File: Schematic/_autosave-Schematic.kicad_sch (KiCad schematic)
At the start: 17 parts, among them Q1 PMOS, Q2 PMOS, Q3 PMOS, Q4 PMOS, Q5 NMOS, Q6 NMOS, Q7 NMOS, Q8 NMOS, U1 TMC262

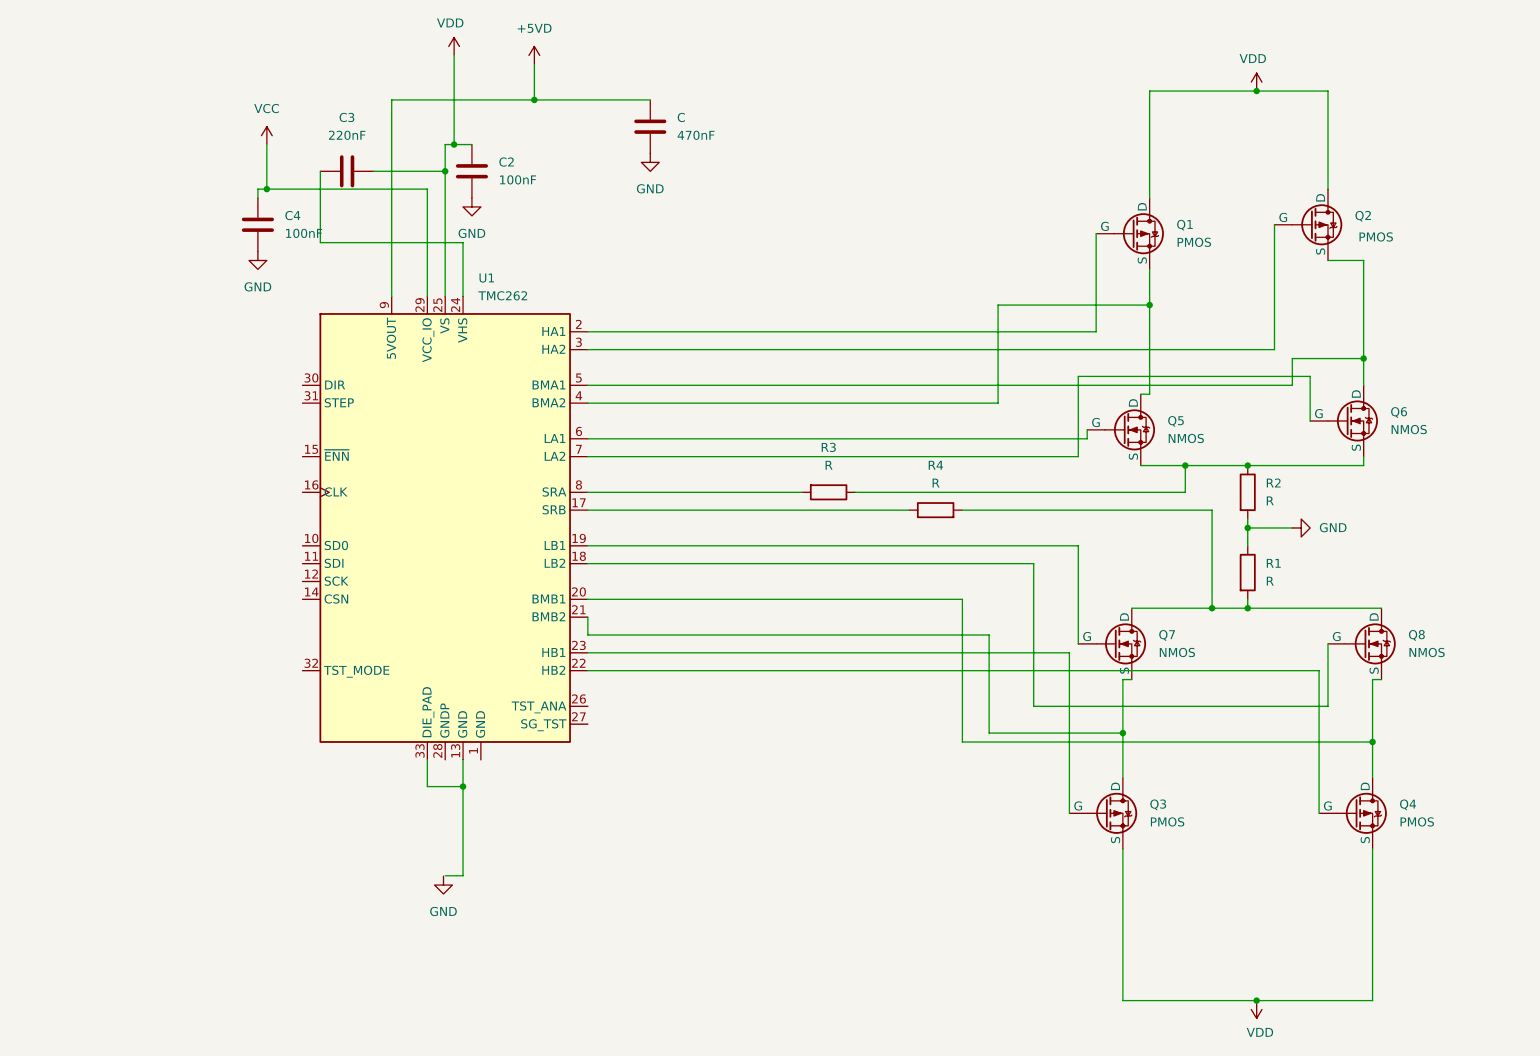
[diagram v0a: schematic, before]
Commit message: working on some stuff
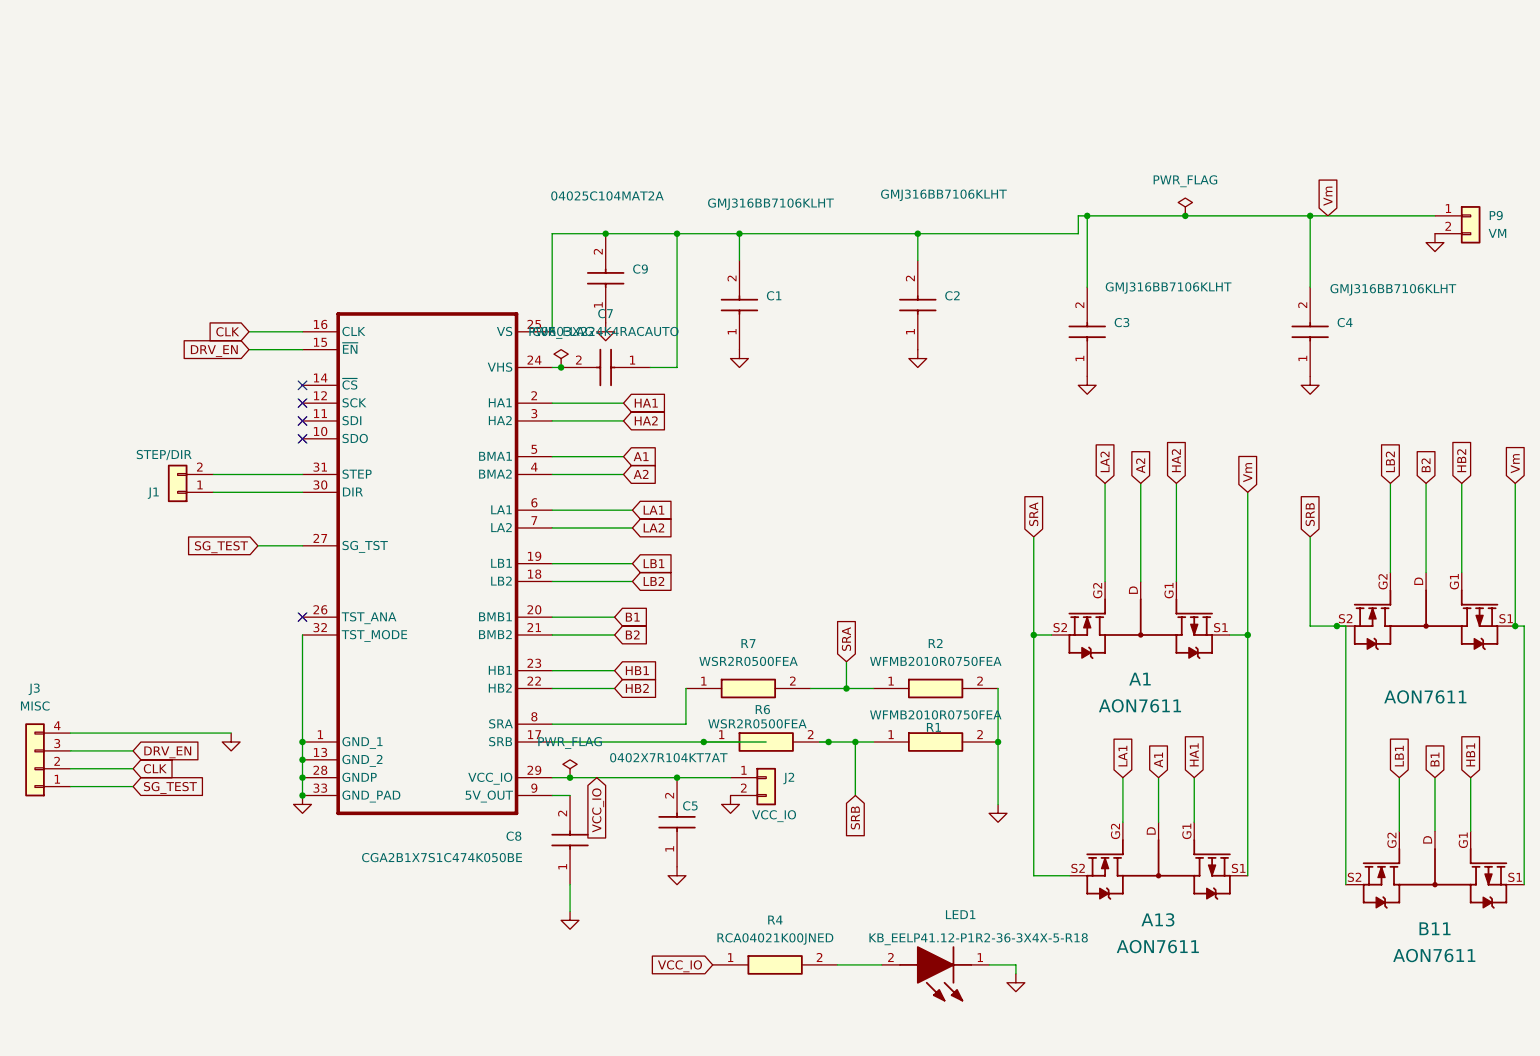
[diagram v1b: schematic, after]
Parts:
- removed C: 470nF, symbol Device:C
- removed C2, C4: 100nF, symbol Device:C
- removed C3: 220nF, symbol Device:C
- removed Q1, Q2, Q3, Q4: PMOS, symbol Simulation_SPICE:PMOS
- removed Q5, Q6, Q7, Q8: NMOS, symbol Simulation_SPICE:NMOS
- removed R1, R2, R3, R4: R, symbol Device:R
- removed U1: TMC262, Package_DFN_QFN:QFN-32-1EP_5x5mm_P0.5mm_EP3.45x3.45mm, symbol Driver_Motor:TMC262
- added A1, A13, B1, B11: AON7611, AON7611, symbol TMC262_BOB40_V1_2:AON7611
- added C1, C2, C3, C4: GMJ316BB7106KLHT, CAPPC3216X125N, symbol GMJ316BB7106KLHT:GMJ316BB7106KLHT
- added C5: 0402X7R104KT7AT, CAPC1005X61N, symbol 0402X7R104KT7AT:0402X7R104KT7AT
- added C7: C0603X224K4RACAUTO, C0603, symbol C0603X224K4RACAUTO:C0603X224K4RACAUTO
- added C8: CGA2B1X7S1C474K050BE, CAPC1005X55N, symbol CGA2B1X7S1C474K050BE:CGA2B1X7S1C474K050BE
- added C9: 04025C104MAT2A, CAPC1005X56N, symbol 04025C104MAT2A:04025C104MAT2A
- added IC1: ~, TMC262-LA:TMC_QFN32_0.5_5.0X5.0, symbol TMC262-LA:TMC262-LA
- added J1: STEP/DIR, symbol Connector_Generic:Conn_01x02
- added J2: VCC_IO, symbol Connector_Generic:Conn_01x02
- added J3: MISC, symbol Connector_Generic:Conn_01x04
- added LED1: KB_EELP41.12-P1R2-36-3X4X-5-R18, KBEELP4112P1R2363X4X5R18, symbol KB_EELP41_12-P1R2-36-3X4X-5-R1:KB_EELP41.12-P1R2-36-3X4X-5-R18
- added P9: VM, symbol Connector_Generic:Conn_01x02
- added R1, R2: WFMB2010R0750FEA, RESC5125X65N, symbol WFMB2010R0750FEA:WFMB2010R0750FEA
- added R4: RCA04021K00JNED, RESC1005X40N, symbol RCA04021K00JNED:RCA04021K00JNED
- added R6, R7: WSR2R0500FEA, RESM11670X254N, symbol WSR2R0500FEA:WSR2R0500FEA
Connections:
- net GND: now also C1.1, C2.1, C3.1, C4.1, C5.1, C8.1, C9.1, IC1.1 (GND_1), IC1.13 (GND_2), IC1.28 (GNDP), IC1.32 (TST_MODE), IC1.33 (GND_PAD), J2.2 (Pin_2), J3.4 (Pin_4), LED1.1 (K), P9.2 (Pin_2), R1.2, R2.2
- new net: C7.2, IC1.24 (VHS)
- new net: IC1.8 (SRA), R7.1
- new net: IC1.17 (SRB), R6.1
- new net: IC1.30 (DIR), J1.1 (Pin_1)
- new net: IC1.31 (STEP), J1.2 (Pin_2)
- new net: C8.2, IC1.9 (5V_OUT)
- new net: LED1.2 (A), R4.2
- new net A1: A13.D, IC1.5 (BMA1)
- new net A2: A1.D, IC1.4 (BMA2)
- new net B1: B11.D, IC1.20 (BMB1)
- new net B2: B1.D, IC1.21 (BMB2)
- new net CLK: IC1.16 (CLK), J3.2 (Pin_2)
- new net DRV_EN: IC1.15 (~{EN}), J3.3 (Pin_3)
- new net HA1: A13.G1, IC1.2 (HA1)
- new net HA2: A1.G1, IC1.3 (HA2)
- new net HB1: B11.G1, IC1.23 (HB1)
- new net HB2: B1.G1, IC1.22 (HB2)
- new net LA1: A13.G2, IC1.6 (LA1)
- new net LA2: A1.G2, IC1.7 (LA2)
- new net LB1: B11.G2, IC1.19 (LB1)
- new net LB2: B1.G2, IC1.18 (LB2)
- new net SG_TEST: IC1.27 (SG_TST), J3.1 (Pin_1)
- new net SRA: A1.S2, A13.S2, R2.1, R7.2
- new net SRB: B1.S2, B11.S2, R1.1, R6.2
- new net VCC_IO: C5.2, IC1.29 (VCC_IO), J2.1 (Pin_1), R4.1
- new net Vm: A1.S1, A13.S1, B1.S1, B11.S1, C1.2, C2.2, C3.2, C4.2, C7.1, C9.2, IC1.25 (VS), P9.1 (Pin_1)
- no-connect marks 0 -> 5
